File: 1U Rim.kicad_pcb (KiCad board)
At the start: 2 copper layers, 56.9 x 28.7 mm, 68 parts, among them J1 Trigger, J10 POT_M, J2 Accent, J3 PWR, J4 Out, J5 PWR_C, J6 PWR_M, J7 JCK_C, J8 JCK_M, J9 POT_C, Q1 BC849, Q2 BC859, Q3 BC849, U1 TL074, U2 TL072

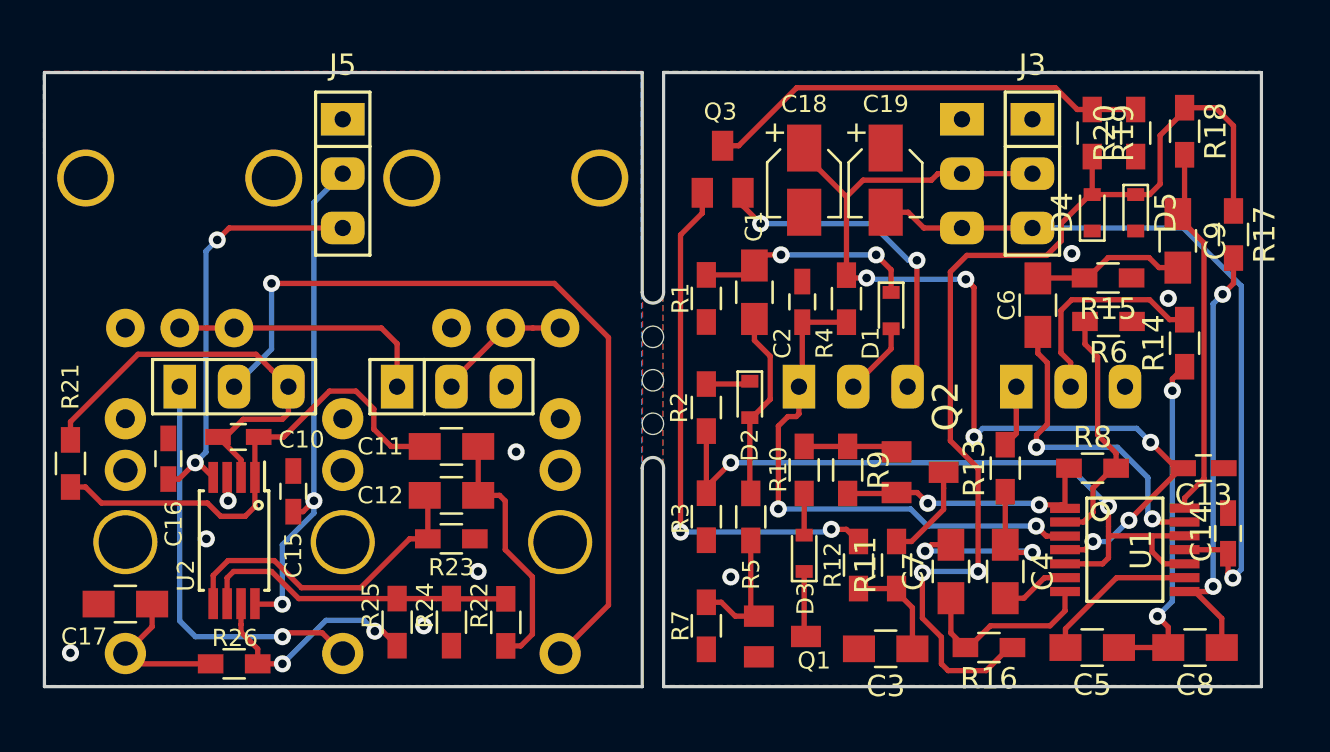
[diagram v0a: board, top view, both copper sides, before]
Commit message: Finished v0.1
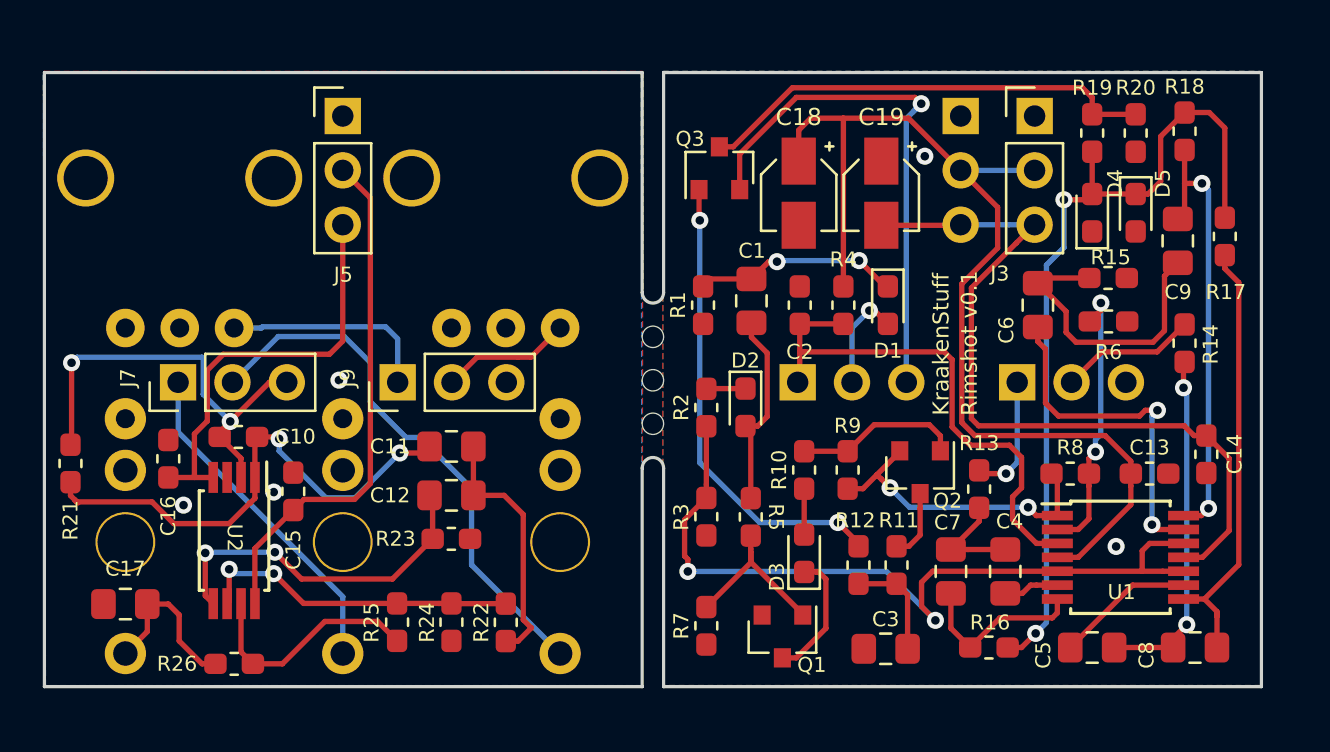
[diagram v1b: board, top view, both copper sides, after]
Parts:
- removed RV1, RV2: A5k, 4ms-footprints:POT-9MM-ALPHA
- added Tune1: A5k, KraakenStuff:POT-9MM-ALPHA, B.Cu at (41.7, 26.6)
- added Tune2: A5k, KraakenStuff:POT-9MM-ALPHA, B.Cu at (26.4, 26.6)
- C1, C11, C12, C17, C3, C4, C5, C6, C7, C8, C9: footprint Capacitors_SMD:C_0805_HandSoldering -> Capacitor_SMD:C_0805_2012Metric_Pad1.15x1.40mm_HandSolder
- C10, C13, C14, C15, C16, C2: footprint Capacitors_SMD:C_0603_HandSoldering -> Capacitor_SMD:C_0603_1608Metric_Pad1.05x0.95mm_HandSolder
- C18, C19: footprint Capacitors_SMD:CP_Elec_3x5.3 -> Capacitor_SMD:CP_Elec_3x5.3
- D1, D2, D3, D4, D5: footprint Diodes_SMD:D_0603 -> Diode_SMD:D_0603_1608Metric_Pad1.05x0.95mm_HandSolder
- J1, J2, J4: footprint 4ms-footprints:PJ301M-12 -> KraakenStuff:PJ301M-12
- J10, J6, J8: footprint MojaBiblioteka:Header 1x3 -> Connector_PinSocket_2.54mm:PinSocket_1x03_P2.54mm_Vertical
- J3, J5, J7, J9: footprint MojaBiblioteka:Header 1x3 -> Connector_PinHeader_2.54mm:PinHeader_1x03_P2.54mm_Vertical
- Q1, Q2, Q3: footprint MojaBiblioteka:SOT23-BCE -> Package_TO_SOT_SMD:SOT-23
- R1, R10, R11, R12, R13, R14, R15, R16, R17, R18, R19, R2, R20, R21, R22, R23, R24, R25, R26, R3, R4, R5, R6, R7, R8, R9: footprint Resistors_SMD:R_0603_HandSoldering -> Resistor_SMD:R_0603_1608Metric_Pad1.05x0.95mm_HandSolder
- U1: footprint SMD_Packages:SSOP-14 -> Package_SO:TSSOP-14_4.4x5mm_P0.65mm
- U2: footprint 4ms-footprints:TSSOP-8_4.4x3mm_Pitch0.65mm -> Package_SO:TSSOP-8_4.4x3mm_P0.65mm
- moved C14 3.83 mm to (74.4, 39.5), turned to 270 degrees
- moved J3 2.69 mm to (66.4, 23.7)
- moved J6 2.69 mm to (62.9, 23.7)
- moved J5 2.69 mm to (34.1, 23.7)
- moved J7 2.62 mm to (26.4, 36.1)
- moved J8 2.61 mm to (55.3, 36.1)
- moved C13 2.53 mm to (71.8, 40.4)
- moved J9 2.52 mm to (36.6, 36.1)
- moved J10 2.51 mm to (65.6, 36.1)
- moved R13 1.56 mm to (63.8, 41.1)
- moved R8 1.07 mm to (68.1, 40.4)
- moved C18 0.66 mm to (55.4, 27.3)
- moved C19 0.64 mm to (59.2, 27.3)
- moved C1 0.43 mm to (53.2, 32.3)
- moved D2 0.42 mm to (52.9, 37.3)
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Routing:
- net Trig: track 41.5 -> 30.3 mm
- net Net-(D4-Pad2): track 50.1 -> 39.8 mm
- net Out: track 36.2 -> 45.5 mm, vias 2 -> 3
- net Net-(C6-Pad1): track 7.14 -> 13.8 mm
- net Net-(C4-Pad1): track 10.3 -> 5.04 mm, vias 2 -> 0
- net Acc: track 44.8 -> 40.6 mm, vias 3 -> 0
- net Ptc2: track 16.5 -> 12.5 mm
- net Net-(R2-Pad1): track 33.9 -> 37.3 mm
- net Net-(Q2-Pad1): track 4.42 -> 7.80 mm
- net +12V: track 71.0 -> 74.3 mm, vias 8 -> 0
- net Net-(C9-Pad1): track 17.5 -> 20.8 mm, vias 0 -> 2
- net Net-(D3-Pad1): track 3.07 -> 6.06 mm
- net Net-(Q3-Pad1): track 24.9 -> 21.9 mm
- net Net-(Q2-Pad2): track 12.4 -> 14.5 mm
- net Net-(Q1-Pad1): track 6.42 -> 8.16 mm
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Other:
- board text added: "KraakenStuff"
- board text added: "Rimshot v0.1"
